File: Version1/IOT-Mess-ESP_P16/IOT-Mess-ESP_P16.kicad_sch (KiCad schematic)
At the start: 23 parts, among them J1 Conn_01x10_Pin, J2 Conn_01x09_Pin, J3 Jumper_2, J4 Jumper_2, J5 Jumper_2, J6 Jumper_2, SW10 SW_Push, SW11 SW_Push, U1 ESP-12F, U10 USB_C_Receptacle_USB2.0_16P, U5 ESP32-C3-WROOM-02, U6 ME6211C33M5

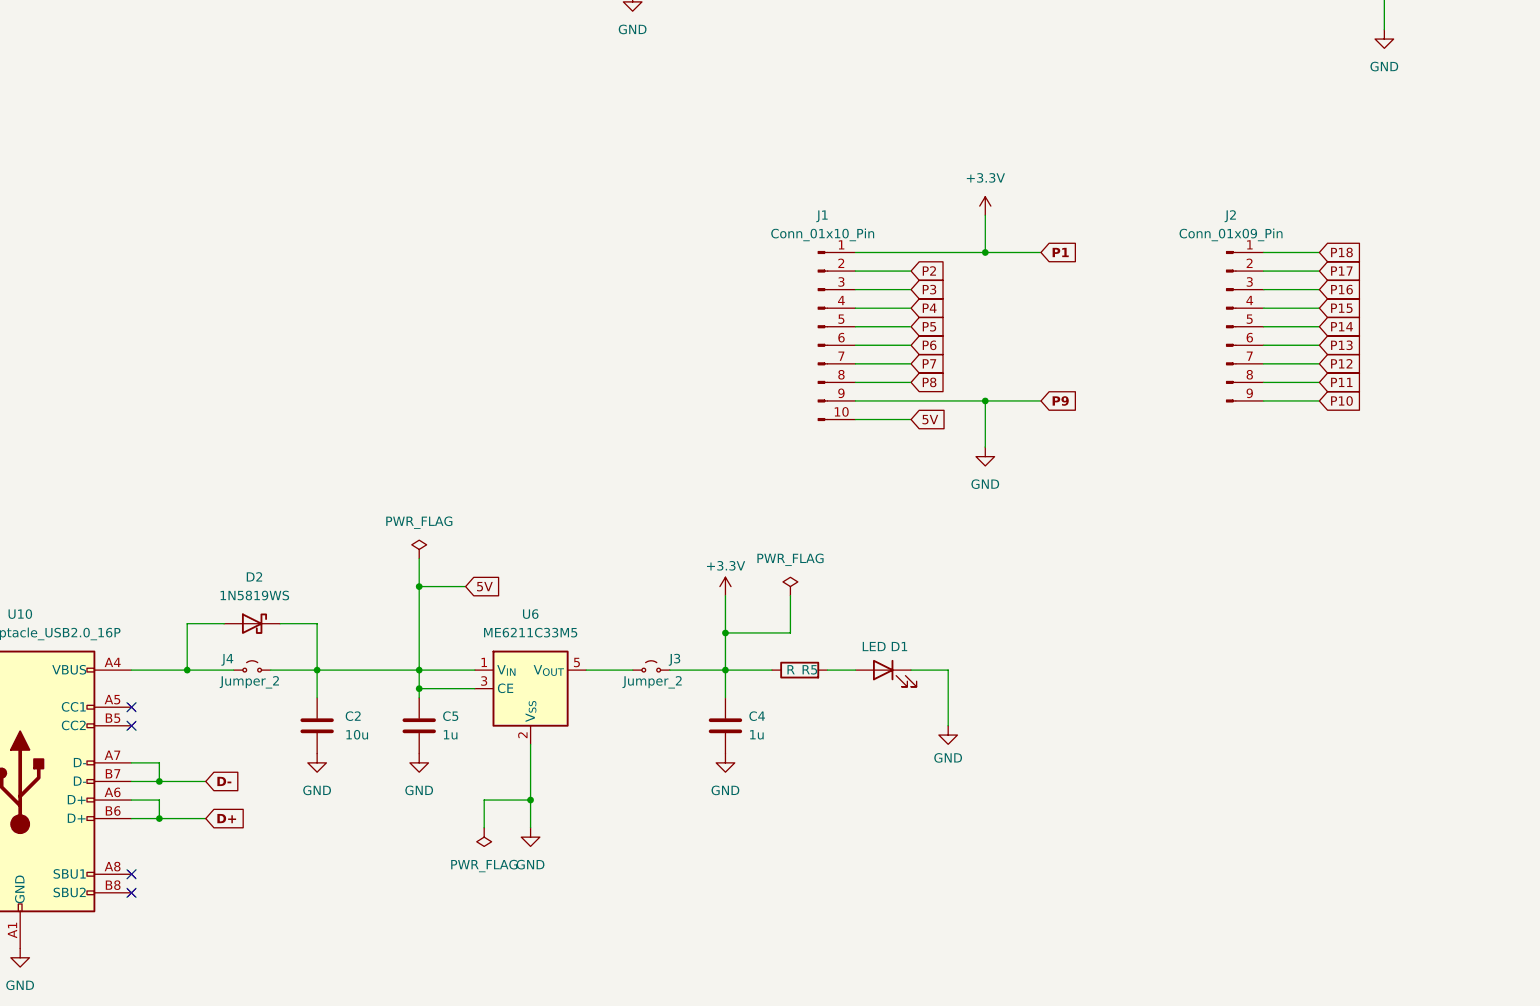
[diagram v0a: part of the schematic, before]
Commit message: updated.
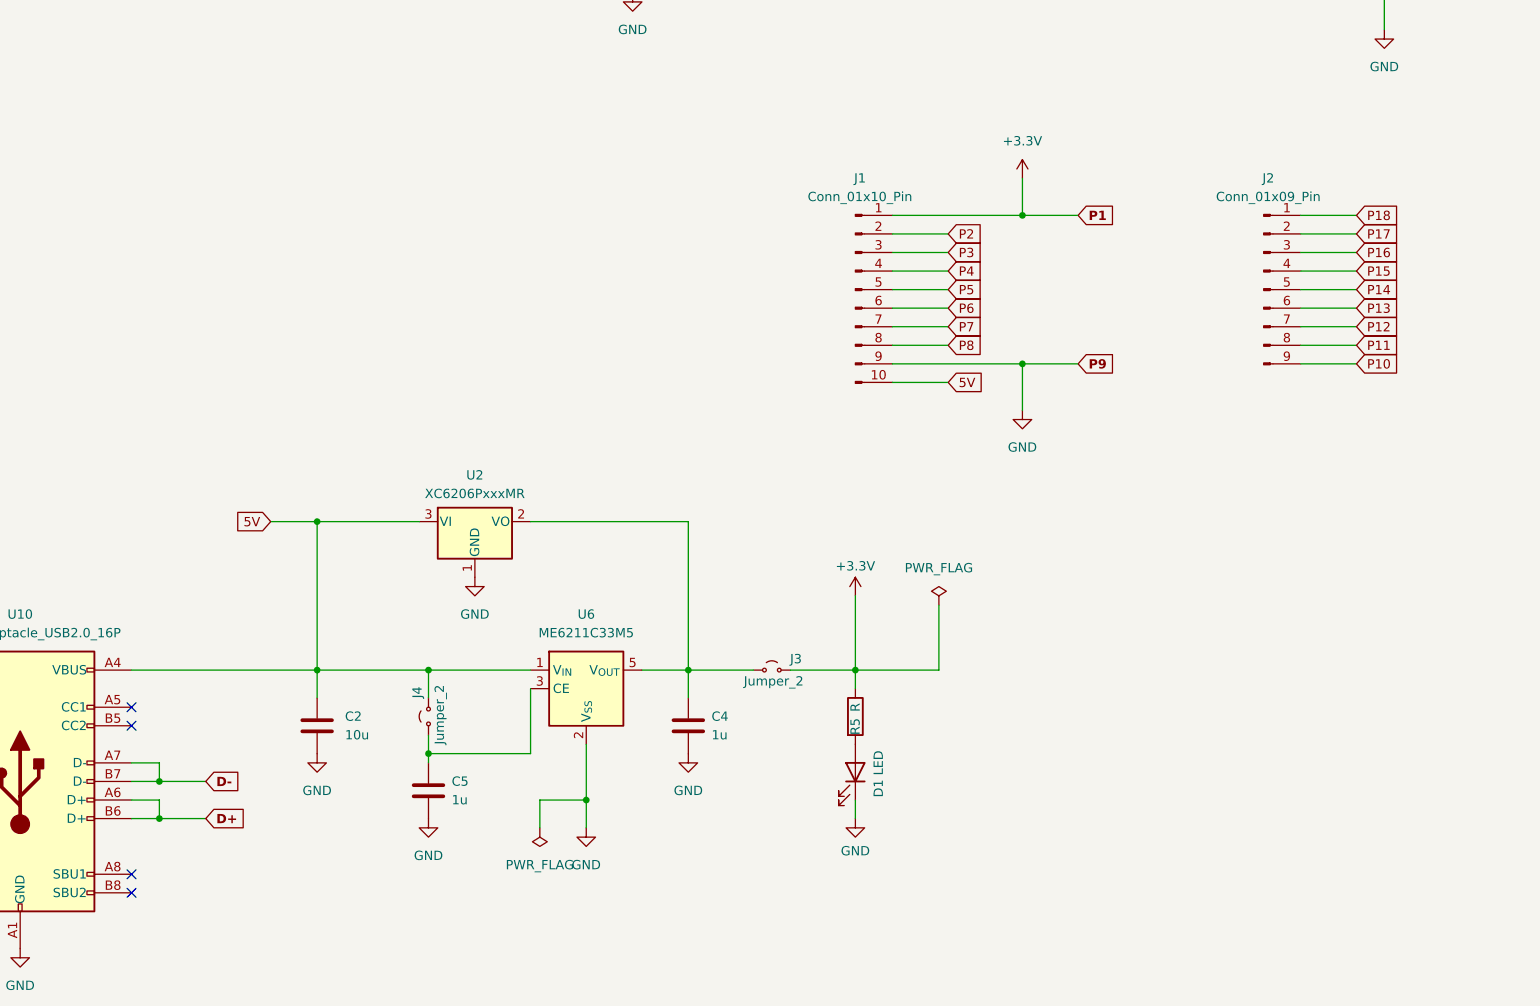
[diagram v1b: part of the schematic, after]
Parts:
- removed D2: 1N5819WS, Diode_SMD:D_SOD-323, symbol Diode:1N5819WS
- added U2: XC6206PxxxMR, Package_TO_SOT_SMD:SOT-23-3, symbol Regulator_Linear:XC6206PxxxMR
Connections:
- net +3.3V: no longer C4.1
- net 5V: now also J4.1 (A), U10.A4 (VBUS), U10.A9 (VBUS), U10.B4 (VBUS), U10.B9 (VBUS), U2.3 (VI); no longer C5.1, J4.2 (B), U6.3 (CE)
- net GND: now also U2.1 (GND)
- net at J3.2 (B), U6.5 (V_{OUT}): now also C4.1, U2.2 (VO)
- new net: C5.1, J4.2 (B), U6.3 (CE)
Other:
- moved on the sheet: C4, C5, D1, J1, J2, J3, R5, U6
